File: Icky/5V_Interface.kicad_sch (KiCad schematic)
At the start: 21 parts, among them IC4 LTC4368IMS-2#PBF, IC7 INA239AQDGSRQ1, Q1102 SOT233 BSS123N, U5 SQJQ112E-T1_GE3, U6 SQJQ112E-T1_GE3

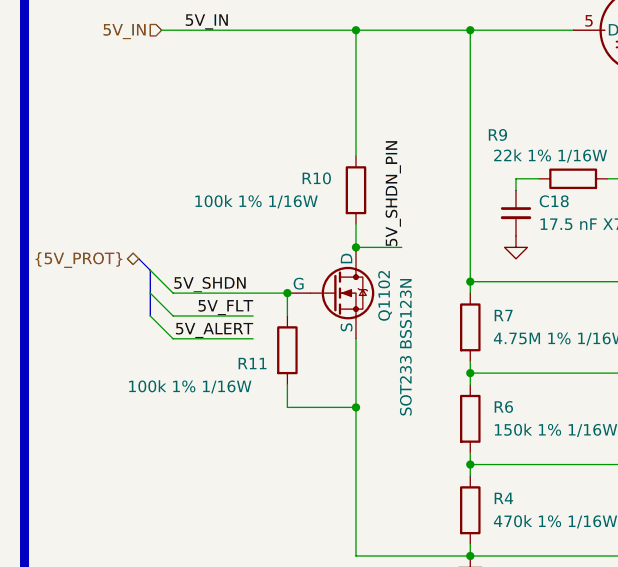
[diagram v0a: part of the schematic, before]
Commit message: ERC passed
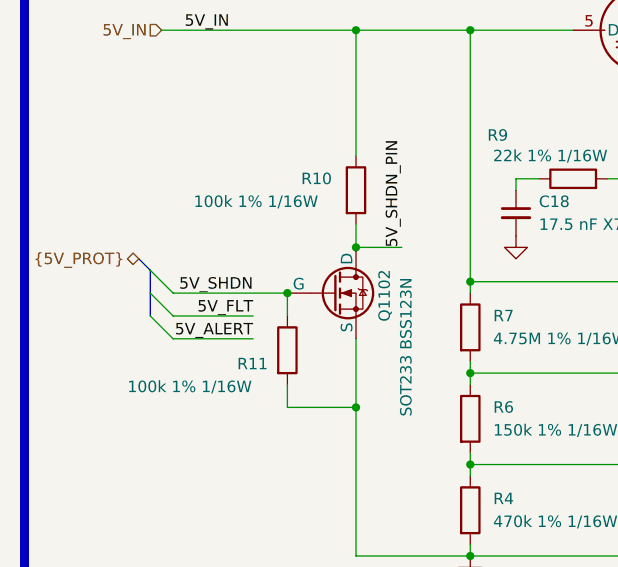
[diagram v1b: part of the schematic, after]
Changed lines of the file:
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@@
 	)
 	(junction
-		(at 49.53 105.41)
+		(at 113.03 76.2)
 		(diameter 0)
 		(color 0 0 0 0)
 	)
 	(junction
-		(at 113.03 76.2)
+		(at 228.6 134.62)
 		(diameter 0)
 		(color 0 0 0 0)
 	)
 	(junction
-		(at 228.6 134.62)
+		(at 229.235 123.19)
 		(diameter 0)
 		(color 0 0 0 0)
 	)
 	(junction
-		(at 229.235 123.19)
+		(at 49.53 105.41)
 		(diameter 0)
 		(color 0 0 0 0)
@@
 	)
 	(bus_entry
-		(at 34.29 107.95)
+		(at 182.245 123.19)
 		(size 2.54 2.54)
 		(stroke
@@
 	)
 	(bus_entry
-		(at 182.245 123.19)
+		(at 182.245 125.73)
 		(size 2.54 2.54)
 		(stroke
@@
 	)
 	(bus_entry
-		(at 182.245 125.73)
+		(at 34.29 105.41)
 		(size 2.54 2.54)
 		(stroke
@@
 	)
 	(bus_entry
-		(at 34.29 102.87)
+		(at 182.245 118.11)
 		(size 2.54 2.54)
 		(stroke
@@
 	)
 	(bus_entry
-		(at 34.29 105.41)
+		(at 34.29 107.95)
 		(size 2.54 2.54)
 		(stroke
@@
 	)
 	(bus_entry
-		(at 182.245 118.11)
+		(at 34.29 102.87)
 		(size 2.54 2.54)
 		(stroke
@@
 	(bus
 		(pts
+			(xy 34.29 102.87) (xy 33.02 101.6)
+		)
+		(stroke
+			(width 0)
+			(type default)
+		)
+	)
+	(bus
+		(pts
 			(xy 182.245 118.11) (xy 182.245 120.65)
 		)
@@
 	(wire
 		(pts
-			(xy 123.19 76.2) (xy 133.35 76.2)
+			(xy 36.83 110.49) (xy 45.72 110.49)
 		)
 		(stroke
@@
 	(wire
 		(pts
-			(xy 137.16 121.92) (xy 137.16 124.46)
+			(xy 123.19 76.2) (xy 133.35 76.2)
 		)
 		(stroke
@@
 	(wire
 		(pts
-			(xy 137.16 104.14) (xy 149.86 104.14)
+			(xy 137.16 121.92) (xy 137.16 124.46)
 		)
 		(stroke
@@
 	(wire
 		(pts
-			(xy 69.85 76.2) (xy 81.28 76.2)
+			(xy 137.16 104.14) (xy 149.86 104.14)
 		)
 		(stroke
@@
 	(wire
 		(pts
-			(xy 91.44 92.71) (xy 95.25 92.71)
+			(xy 69.85 76.2) (xy 81.28 76.2)
 		)
 		(stroke
@@
 	(wire
 		(pts
-			(xy 184.785 125.73) (xy 196.85 125.73)
+			(xy 91.44 92.71) (xy 95.25 92.71)
 		)
 		(stroke
@@
 		)
 	)
-	(bus
+	(wire
 		(pts
-			(xy 34.29 102.87) (xy 34.29 105.41)
+			(xy 184.785 125.73) (xy 196.85 125.73)
 		)
 		(stroke
@@
 		)
 	)
-	(bus
+	(wire
 		(pts
-			(xy 34.29 102.87) (xy 33.02 101.6)
+			(xy 36.83 107.95) (xy 45.72 107.95)
 		)
 		(stroke
@@
 	(wire
 		(pts
-			(xy 57.15 100.33) (xy 62.23 100.33)
+			(xy 36.83 105.41) (xy 49.53 105.41)
 		)
 		(stroke
@@
 	(wire
 		(pts
-			(xy 95.25 90.17) (xy 95.25 92.71)
+			(xy 57.15 100.33) (xy 62.23 100.33)
 		)
 		(stroke
@@
 	(wire
 		(pts
-			(xy 247.65 123.19) (xy 254 123.19)
+			(xy 95.25 90.17) (xy 95.25 92.71)
 		)
 		(stroke
@@
 	(wire
 		(pts
-			(xy 228.6 135.89) (xy 228.6 134.62)
+			(xy 247.65 123.19) (xy 254 123.19)
 		)
 		(stroke
@@
 	(wire
 		(pts
-			(xy 36.83 107.95) (xy 45.72 107.95)
+			(xy 228.6 135.89) (xy 228.6 134.62)
 		)
 		(stroke
@@
 		)
 	)
-	(wire
-		(pts
-			(xy 36.83 110.49) (xy 45.72 110.49)
-		)
-		(stroke
-			(width 0)
-			(type default)
-		)
-	)
 	(bus
 		(pts
@@
 		)
 	)
-	(wire
+	(bus
 		(pts
-			(xy 121.92 76.2) (xy 123.19 76.2)
+			(xy 34.29 102.87) (xy 34.29 105.41)
 		)
 		(stroke
@@
 	(wire
 		(pts
-			(xy 57.15 97.79) (xy 57.15 100.33)
+			(xy 121.92 76.2) (xy 123.19 76.2)
 		)
 		(stroke
@@
 	(wire
 		(pts
-			(xy 229.235 123.19) (xy 229.235 125.73)
+			(xy 57.15 97.79) (xy 57.15 100.33)
 		)
 		(stroke
@@
 	(wire
 		(pts
-			(xy 69.85 134.62) (xy 137.16 134.62)
+			(xy 229.235 123.19) (xy 229.235 125.73)
 		)
 		(stroke
@@
 	(wire
 		(pts
-			(xy 102.87 91.44) (xy 102.87 92.71)
+			(xy 69.85 134.62) (xy 137.16 134.62)
 		)
 		(stroke
@@
 	(wire
 		(pts
-			(xy 36.83 105.41) (xy 49.53 105.41)
+			(xy 102.87 91.44) (xy 102.87 92.71)
 		)
 		(stroke
@@
 		)
 	)
-	(label "SPI1_SCK"
-		(at 184.785 128.27 0)
+	(label "5V_ALERT"
+		(at 45.72 110.49 180)
 		(effects
 			(font
 				(size 1.27 1.27)
 			)
-			(justify left bottom)
+			(justify right bottom)
 		)
 	)
-	(label "5V_OUT"
-		(at 124.46 76.2 0)
+	(label "SPI1_SCK"
+		(at 184.785 128.27 0)
 		(effects
 			(font
@@
 		)
 	)
-	(label "5V_D"
-		(at 254 120.65 0)
+	(label "5V_SHDN"
+		(at 45.72 105.41 180)
 		(effects
 			(font
 				(size 1.27 1.27)
 			)
-			(justify left bottom)
+			(justify right bottom)
 		)
 	)
-	(label "5V_D"
-		(at 113.03 90.17 0)
+	(label "5V_OUT"
+		(at 124.46 76.2 0)
 		(effects
 			(font
@@
 		)
 	)
-	(label "5V_SHDN_PIN"
-		(at 62.23 100.33 90)
+	(label "5V_D"
+		(at 254 120.65 0)
 		(effects
 			(font
@@
 		)
 	)
-	(label "5V_ALERT"
-		(at 184.15 130.81 0)
+	(label "5V_D"
+		(at 113.03 90.17 0)
 		(effects
 			(font
@@
 		)
 	)
-	(label "5V_SHDN"
-		(at 36.83 105.41 0)
+	(label "5V_SHDN_PIN"
+		(at 62.23 100.33 90)
 		(effects
 			(font
@@
 	)
 	(label "5V_ALERT"
-		(at 45.72 110.49 180)
+		(at 184.15 130.81 0)
 		(effects
 			(font
 				(size 1.27 1.27)
 			)
-			(justify right bottom)
+			(justify left bottom)
 		)
 	)
@@
 		)
 	)
-	(hierarchical_label "5V_IN"
-		(shape input)
-		(at 35.56 76.2 180)
+	(hierarchical_label "{5V_PROT}"
+		(shape bidirectional)
+		(at 33.02 101.6 180)
 		(effects
 			(font
@@
 		)
 	)
-	(hierarchical_label "{5V_PROT}"
-		(shape bidirectional)
-		(at 33.02 101.6 180)
+	(hierarchical_label "5V_IN"
+		(shape input)
+		(at 35.56 76.2 180)
 		(effects
 			(font
